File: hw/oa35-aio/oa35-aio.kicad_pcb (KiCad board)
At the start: 6 copper layers, 36 x 36 mm, 283 parts, among them J1 TYPE-C-31-M-12, J10 M1A, J11 M1B, J12 M1C, J13 M2A, J14 M2B, J15 M2C, J16 M3A, J17 M3B, J18 M3C, J19 M4A, J2 SM06B-SRSS-TB, J20 M4B, J21 M4C, J3 BAT+, J4 BAT-, P1 +5V, P10 TX6, P11 RX1, P12 TX1, P13 LED, P14 BZ-, P15 BZ+, P16 RSSI, P17 SCL, P18 SDA, P19 +3V3, P2 GND, P20 GND, P21 VBAT, P22 GND, P3 RX2, P4 TX2, P5 +5V, P6 GND, P7 RX4, P8 TX4, P9 RX6, Q1 2N7002, U1 INA186A3IDCKR, U10 USBLC6-2SC6, U2 LMR51430YFDDCR, U20 AT32F421G8U7, U21 NSG2065Q, U3 LMR51430YFDDCR, U30 AT32F421G8U7, U31 NSG2065Q, U4 LP5912-3.3DRVR, U40 AT32F421G8U7, U41 NSG2065Q, U5 TLV76733DRVR, U50 AT32F421G8U7, U51 NSG2065Q, U6 STM32F722RET6, U7 ICM-42688-P, U8 BMP280, U9 W25Q128JVSIQ, Y1 8MHz

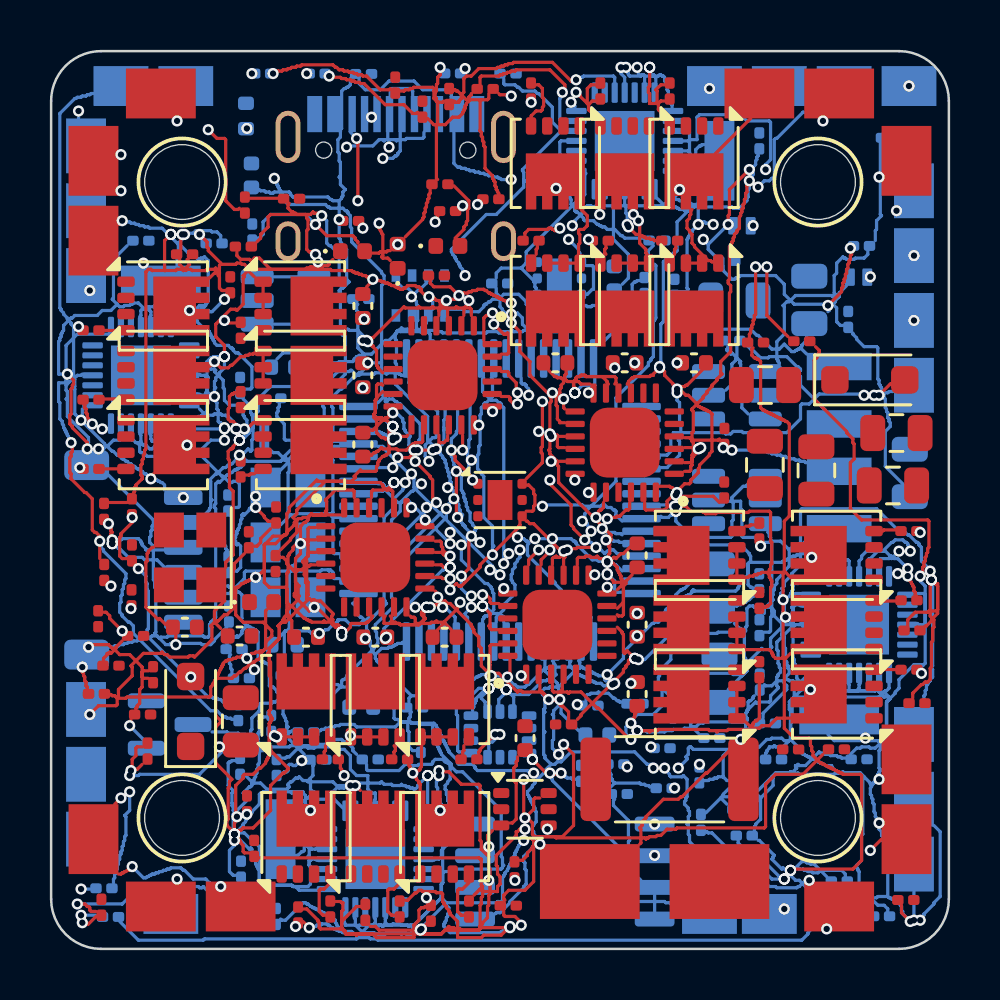
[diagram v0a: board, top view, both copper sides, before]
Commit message: OA35-AIO: routing iteration 3
Co-Authored-By: Claude Opus 5 <noreply@anthropic.com>
Claude-Session: https://claude.ai/code/session_013J1rgXZWykCJN7jVVS67P2
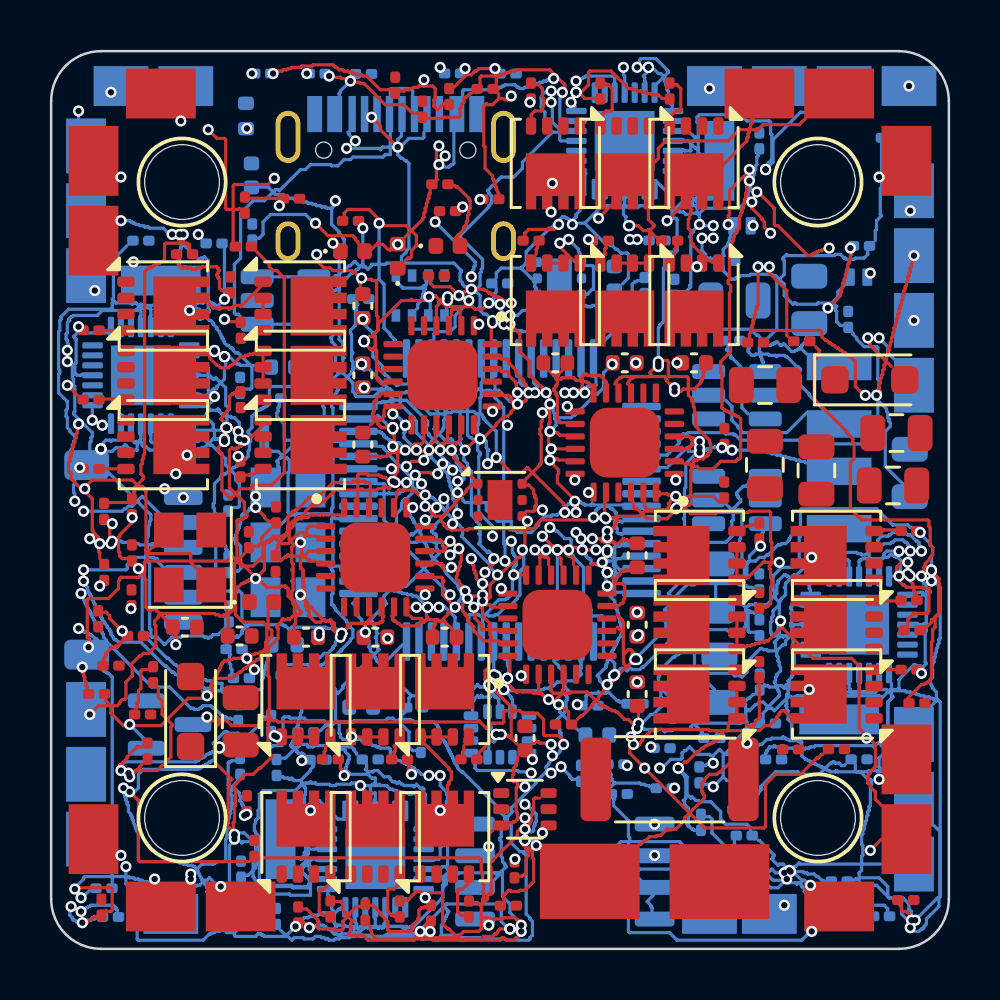
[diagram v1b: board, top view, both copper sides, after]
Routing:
- net UART2_RX: track 45.1 -> 60.3 mm, vias 3 -> 4
- net NRST_4: track 18.6 -> 31.0 mm, vias 2 -> 3
- net LED1: track 18.6 -> 30.5 mm, vias 1 -> 2
- net PH_B_3: track 29.4 -> 41.0 mm
- net FBB_1: track 34.8 -> 45.0 mm, vias 1 -> 3
- net BL_3: track 24.5 -> 34.2 mm
- net FBA_3: track 29.6 -> 39.2 mm
- net HSE_IN: track 19.0 -> 28.4 mm
- net PH_B_4: track 54.2 -> 44.9 mm
- net PH_C_1: track 33.2 -> 42.2 mm, vias 4 -> 5
- net CC2: track 26.7 -> 35.7 mm, vias 3 -> 2
- net BOOTA_3: track 11.5 -> 20.3 mm, vias 0 -> 2
- net UART1_TX: track 37.3 -> 45.7 mm
- net FLASH_MOSI: track 9.35 -> 17.6 mm
- net PH_C_2: track 57.3 -> 64.6 mm, vias 4 -> 6
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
